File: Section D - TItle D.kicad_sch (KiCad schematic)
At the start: 0 parts

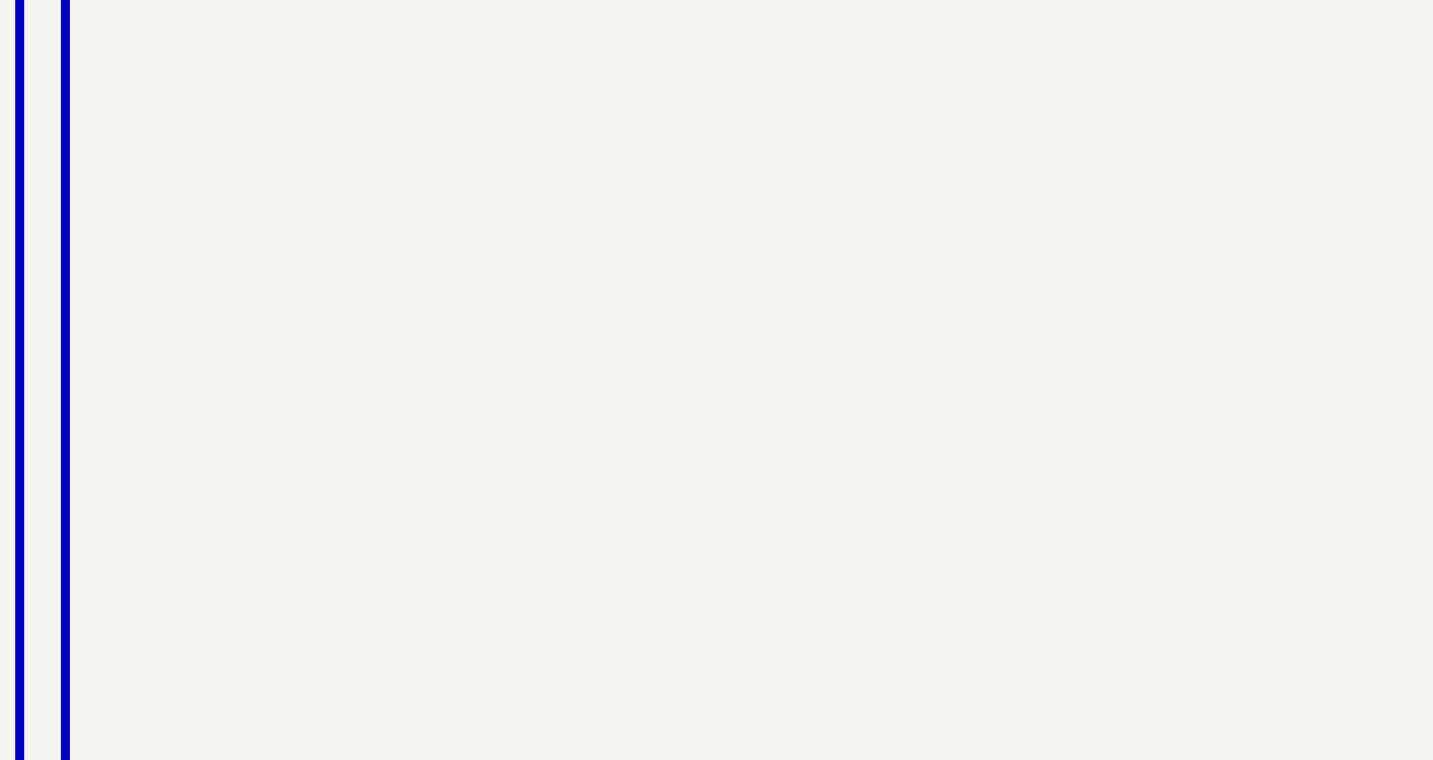
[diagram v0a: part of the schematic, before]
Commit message: [Finish schématique]
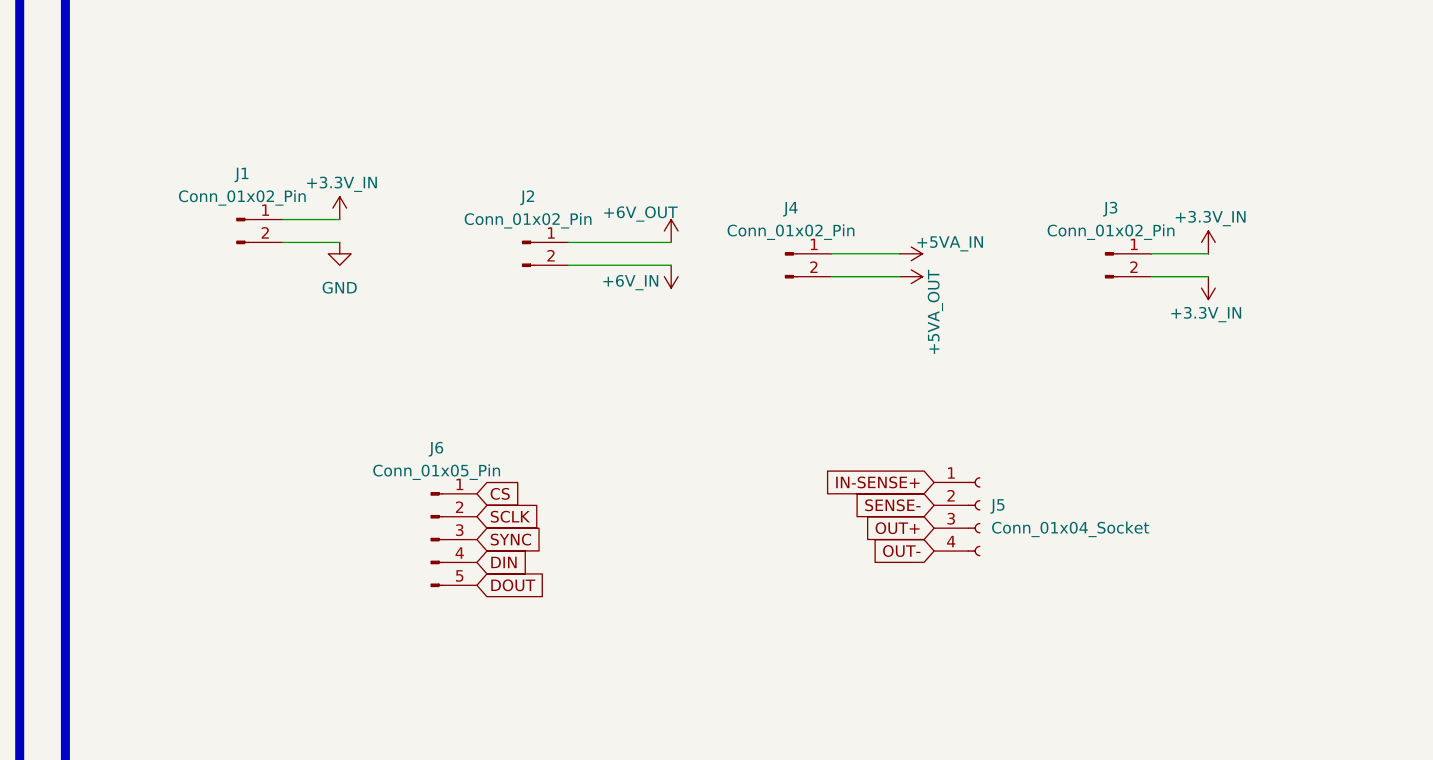
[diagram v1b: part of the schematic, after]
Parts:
- added J1, J2, J3, J4: Conn_01x02_Pin, Connector_PinHeader_2.54mm:PinHeader_1x02_P2.54mm_Vertical, symbol Connector:Conn_01x02_Pin
- added J5: Conn_01x04_Socket, Connector_PinSocket_2.54mm:PinSocket_1x04_P2.54mm_Vertical, symbol Connector:Conn_01x04_Socket
- added J6: Conn_01x05_Pin, Connector_PinSocket_2.54mm:PinSocket_1x05_P2.54mm_Vertical, symbol Connector:Conn_01x05_Pin
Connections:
- new net +3.3V_IN: J1.1 (Pin_1), J3.1 (Pin_1), J3.2 (Pin_2)
- new net +5VA_IN: J4.1 (Pin_1)
- new net +5VA_OUT: J4.2 (Pin_2)
- new net +6V_IN: J2.2 (Pin_2)
- new net +6V_OUT: J2.1 (Pin_1)
- new net CS: J6.1 (Pin_1)
- new net DIN: J6.4 (Pin_4)
- new net DOUT: J6.5 (Pin_5)
- new net GND: J1.2 (Pin_2)
- new net IN-SENSE+: J5.1 (Pin_1)
- new net OUT+: J5.3 (Pin_3)
- new net OUT-: J5.4 (Pin_4)
- new net SCLK: J6.2 (Pin_2)
- new net SENSE-: J5.2 (Pin_2)
- new net SYNC: J6.3 (Pin_3)

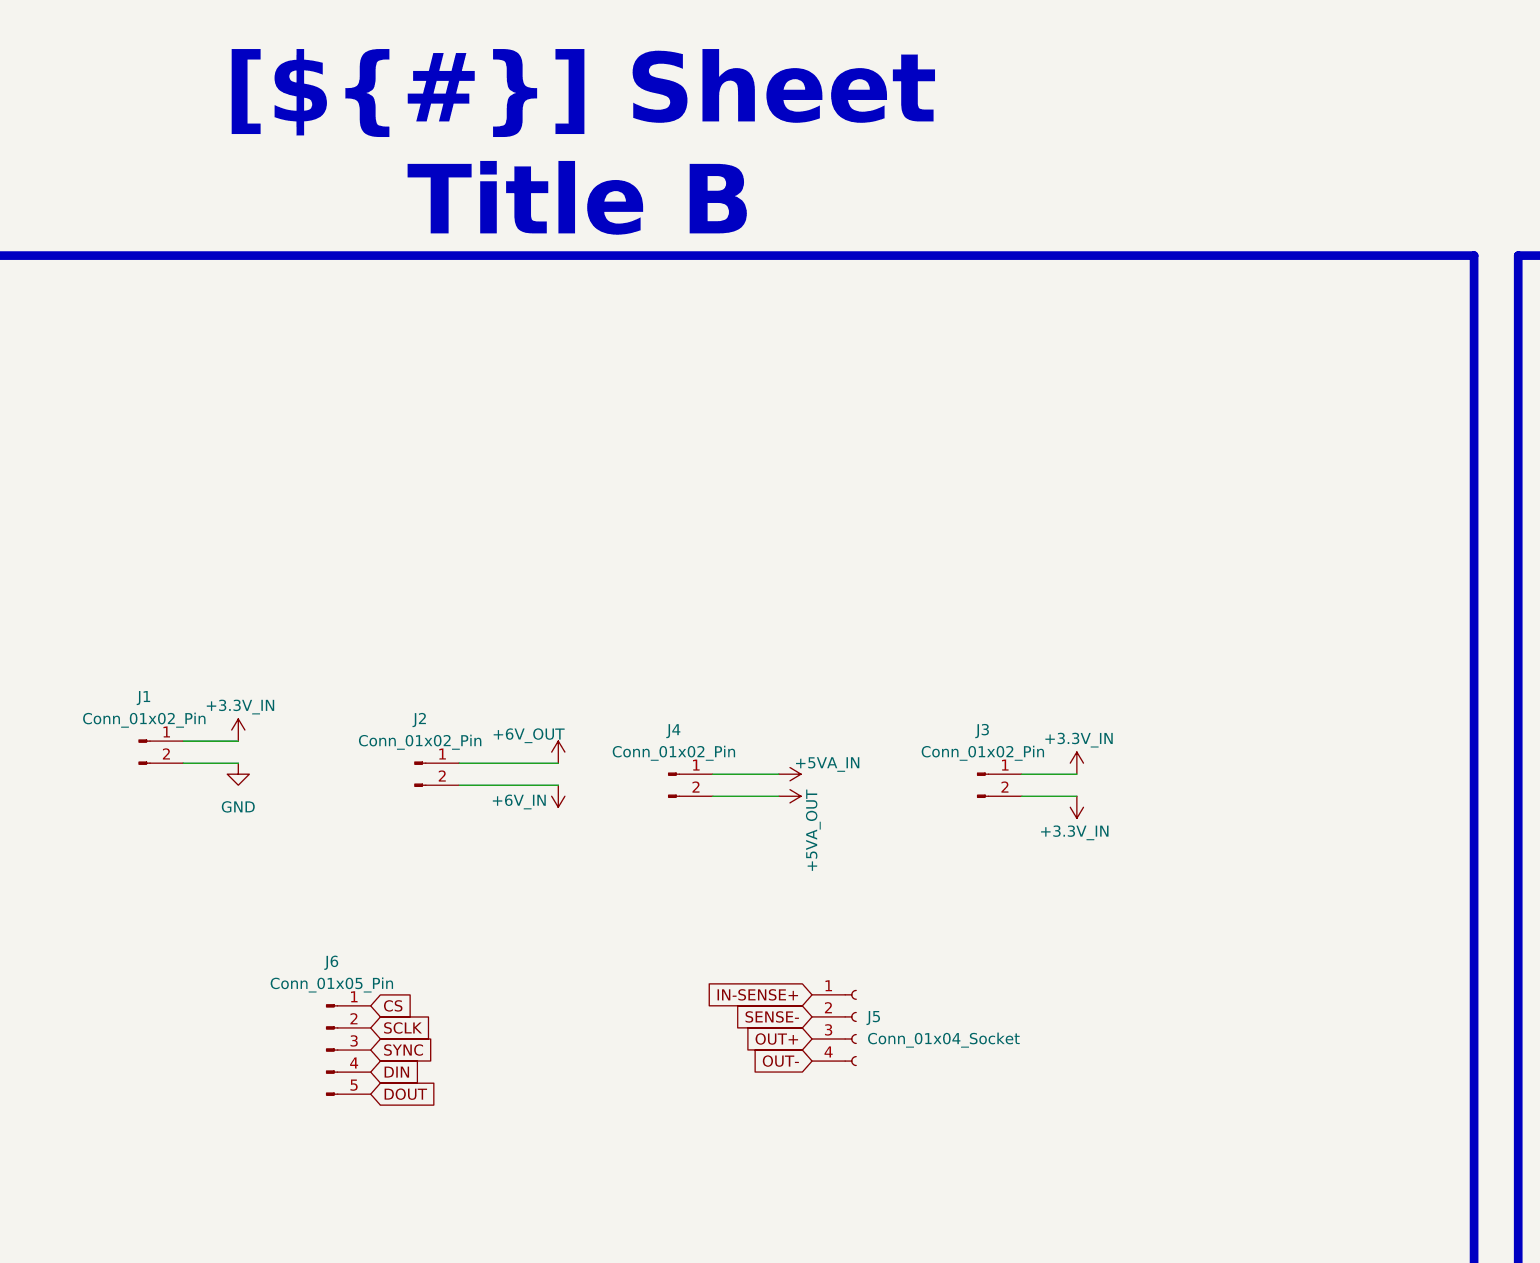
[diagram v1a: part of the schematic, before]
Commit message: [Finish schématiq]
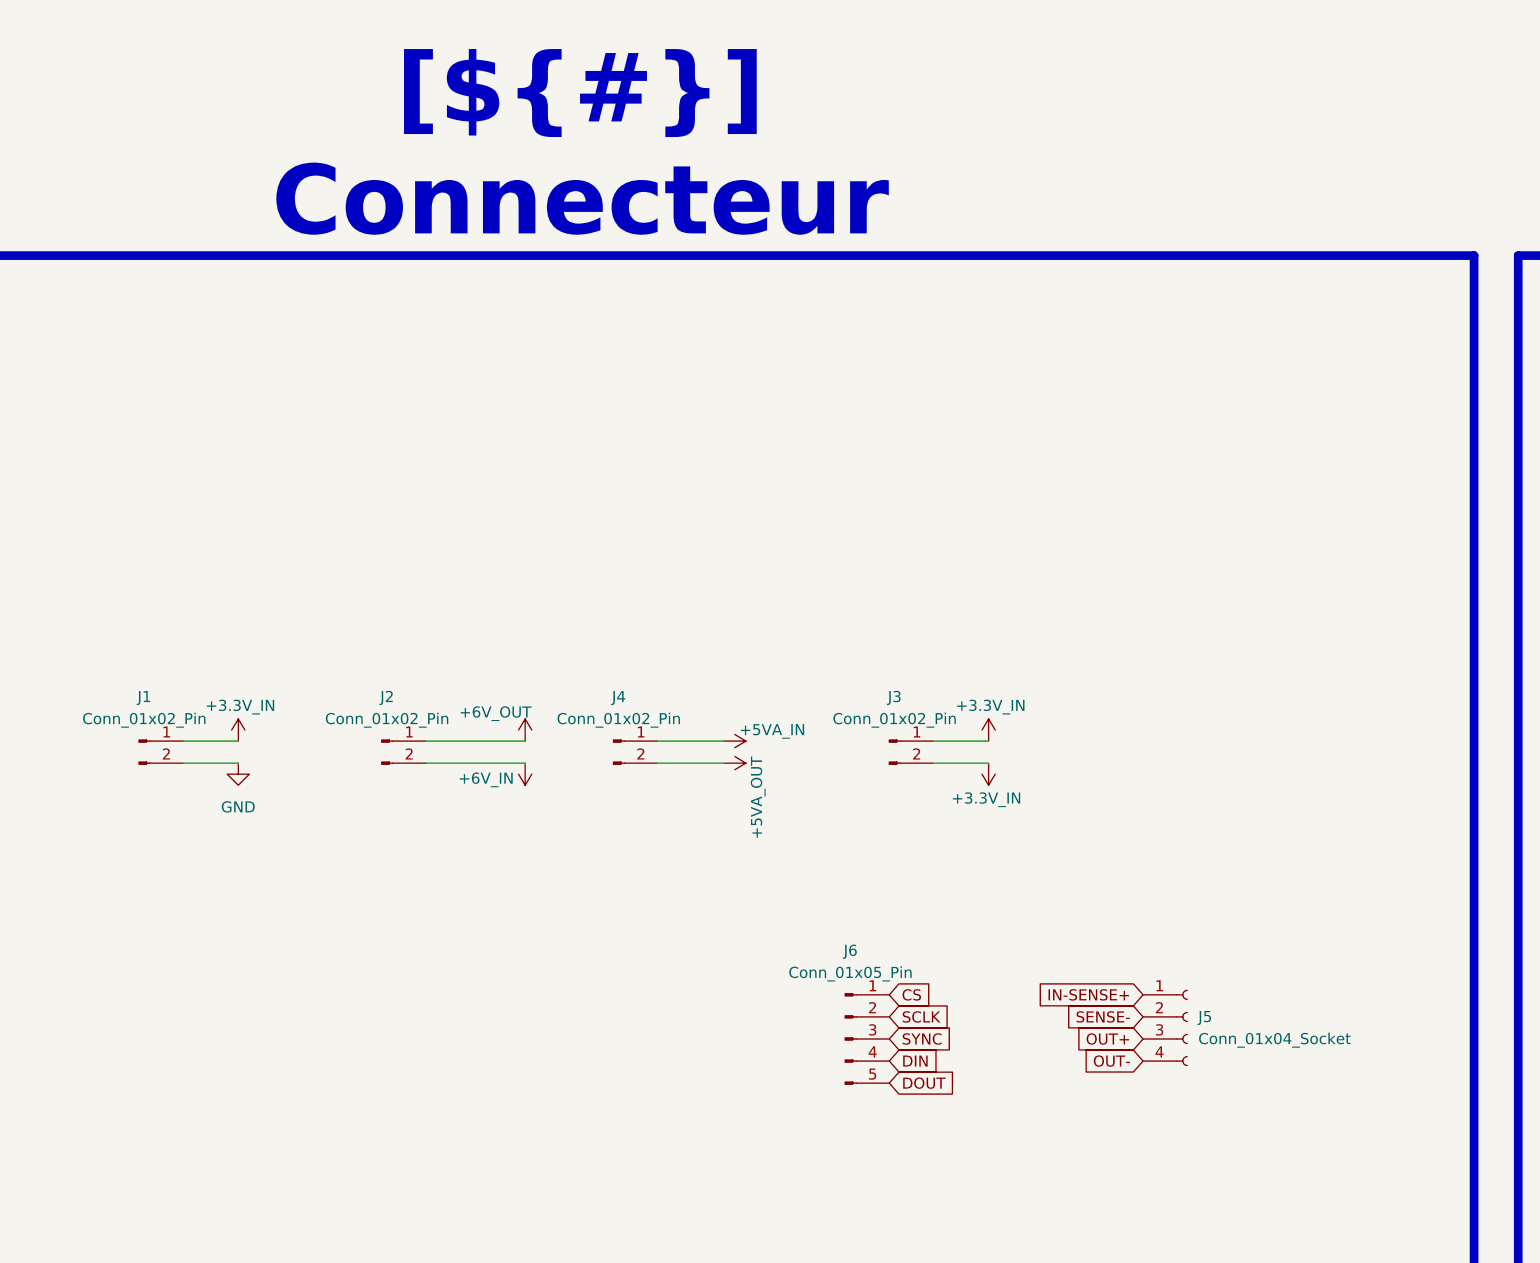
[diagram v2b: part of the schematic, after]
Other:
- moved on the sheet: J2, J3, J4, J5, J6

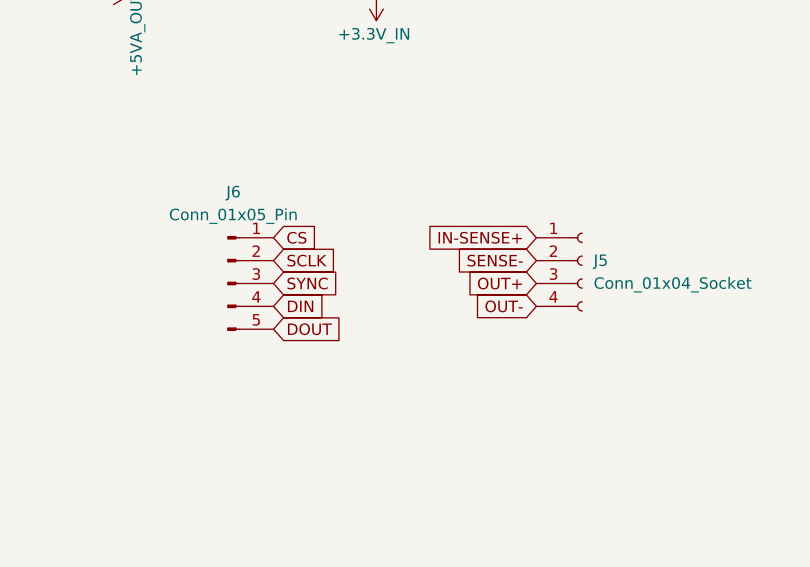
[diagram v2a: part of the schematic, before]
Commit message: [PCB fini]
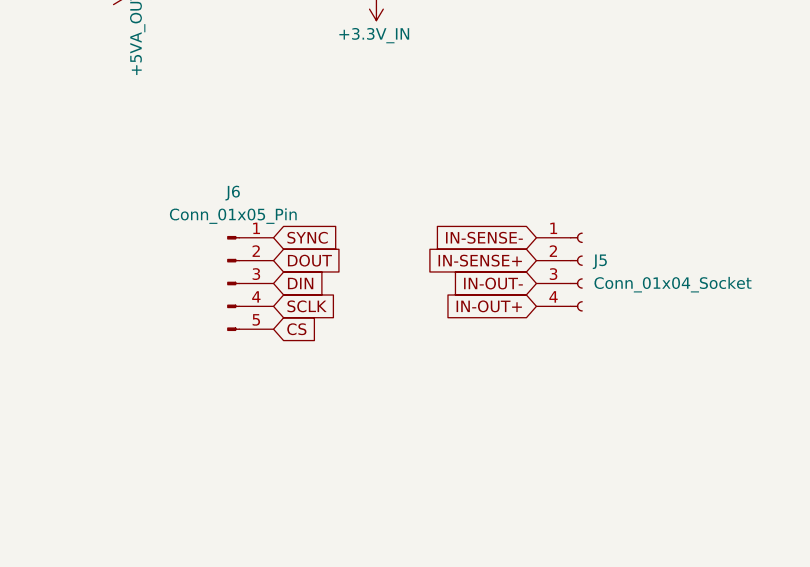
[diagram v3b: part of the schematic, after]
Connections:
- net SENSE- is gone; now on net IN-SENSE+: J5.2 (Pin_2)
- net CS: now also J6.5 (Pin_5); no longer J6.1 (Pin_1)
- net DIN: now also J6.3 (Pin_3); no longer J6.4 (Pin_4)
- net DOUT: now also J6.2 (Pin_2); no longer J6.5 (Pin_5)
- net IN-SENSE+: no longer J5.1 (Pin_1)
- net SCLK: now also J6.4 (Pin_4); no longer J6.2 (Pin_2)
- net SYNC: now also J6.1 (Pin_1); no longer J6.3 (Pin_3)
- net OUT+ renamed IN-OUT-
- net OUT- renamed IN-OUT+
- new net IN-SENSE-: J5.1 (Pin_1)
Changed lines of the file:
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@@
 		)
 	)
-	(global_label "SCLK"
+	(global_label "CS"
 		(shape input)
-		(at 245.11 127 0)
+		(at 245.11 134.62 0)
 		(fields_autoplaced yes)
 		(effects
@@
 		)
 		(property "Intersheetrefs" "${INTERSHEET_REFS}"
-			(at 252.8728 127 0)
+			(at 250.5747 134.62 0)
 			(effects
 				(font
@@
 		)
 	)
-	(global_label "CS"
+	(global_label "IN-OUT-"
 		(shape input)
-		(at 245.11 124.46 0)
+		(at 274.32 129.54 180)
+		(fields_autoplaced yes)
+		(effects
+			(font
+				(size 1.27 1.27)
+			)
+			(justify right)
+		)
+		(property "Intersheetrefs" "${INTERSHEET_REFS}"
+			(at 262.6261 129.54 0)
+			(effects
+				(font
+					(size 1.27 1.27)
+				)
+				(justify right)
+				(hide yes)
+			)
+		)
+	)
+	(global_label "DIN"
+		(shape input)
+		(at 245.11 129.54 0)
 		(fields_autoplaced yes)
 		(effects
@@
 		)
 		(property "Intersheetrefs" "${INTERSHEET_REFS}"
-			(at 250.5747 124.46 0)
+			(at 251.3005 129.54 0)
 			(effects
 				(font
@@
 		)
 	)
-	(global_label "IN-SENSE+"
+	(global_label "IN-SENSE-"
 		(shape input)
 		(at 274.32 124.46 180)
@@
 		)
 	)
-	(global_label "OUT-"
+	(global_label "DOUT"
+		(shape input)
+		(at 245.11 127 0)
+		(fields_autoplaced yes)
+		(effects
+			(font
+				(size 1.27 1.27)
+			)
+			(justify left)
+		)
+		(property "Intersheetrefs" "${INTERSHEET_REFS}"
+			(at 252.9938 127 0)
+			(effects
+				(font
+					(size 1.27 1.27)
+				)
+				(justify left)
+				(hide yes)
+			)
+		)
+	)
+	(global_label "IN-OUT+"
 		(shape input)
 		(at 274.32 132.08 180)
@@
 		)
 		(property "Intersheetrefs" "${INTERSHEET_REFS}"
-			(at 266.1338 132.08 0)
+			(at 262.6261 132.08 0)
 			(effects
 				(font
@@
 		)
 	)
-	(global_label "SENSE-"
+	(global_label "SCLK"
+		(shape input)
+		(at 245.11 132.08 0)
+		(fields_autoplaced yes)
+		(effects
+			(font
+				(size 1.27 1.27)
+			)
+			(justify left)
+		)
+		(property "Intersheetrefs" "${INTERSHEET_REFS}"
+			(at 252.8728 132.08 0)
+			(effects
+				(font
+					(size 1.27 1.27)
+				)
+				(justify left)
+				(hide yes)
+			)
+		)
+	)
+	(global_label "IN-SENSE+"
 		(shape input)
 		(at 274.32 127 180)
@@
 		)
 		(property "Intersheetrefs" "${INTERSHEET_REFS}"
-			(at 263.7149 127 0)
-			(effects
-				(font
-					(size 1.27 1.27)
-				)
-				(justify right)
-				(hide yes)
-			)
-		)
-	)
-	(global_label "OUT+"
-		(shape input)
-		(at 274.32 129.54 180)
-		(fields_autoplaced yes)
-		(effects
-			(font
-				(size 1.27 1.27)
-			)
-			(justify right)
-		)
-		(property "Intersheetrefs" "${INTERSHEET_REFS}"
-			(at 266.1338 129.54 0)
+			(at 260.2072 127 0)
 			(effects
 				(font
@@
 	(global_label "SYNC"
 		(shape input)
-		(at 245.11 129.54 0)
+		(at 245.11 124.46 0)
 		(fields_autoplaced yes)
 		(effects
@@
 		)
 		(property "Intersheetrefs" "${INTERSHEET_REFS}"
-			(at 252.9938 129.54 0)
+			(at 252.9938 124.46 0)
 			(effects
 				(font
-					(size 1.27 1.27)
-				)
-				(justify left)
-				(hide yes)
-			)
-		)
-	)
-	(global_label "DIN"
-		(shape input)
-		(at 245.11 132.08 0)
-		(fields_autoplaced yes)
-		(effects
-			(font
-				(size 1.27 1.27)
-			)
-			(justify left)
-		)
-		(property "Intersheetrefs" "${INTERSHEET_REFS}"
-			(at 251.3005 132.08 0)
-			(effects
-				(font
-					(size 1.27 1.27)
-				)
-				(justify left)
-				(hide yes)
-			)
-		)
-	)
-	(global_label "DOUT"
-		(shape input)
-		(at 245.11 134.62 0)
-		(fields_autoplaced yes)
-		(effects
-			(font
-				(size 1.27 1.27)
-			)
-			(justify left)
-		)
-		(property "Intersheetrefs" "${INTERSHEET_REFS}"
-			(at 252.9938 134.62 0)
-			(effects
-				(font
